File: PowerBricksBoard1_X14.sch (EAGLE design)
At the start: 16 parts

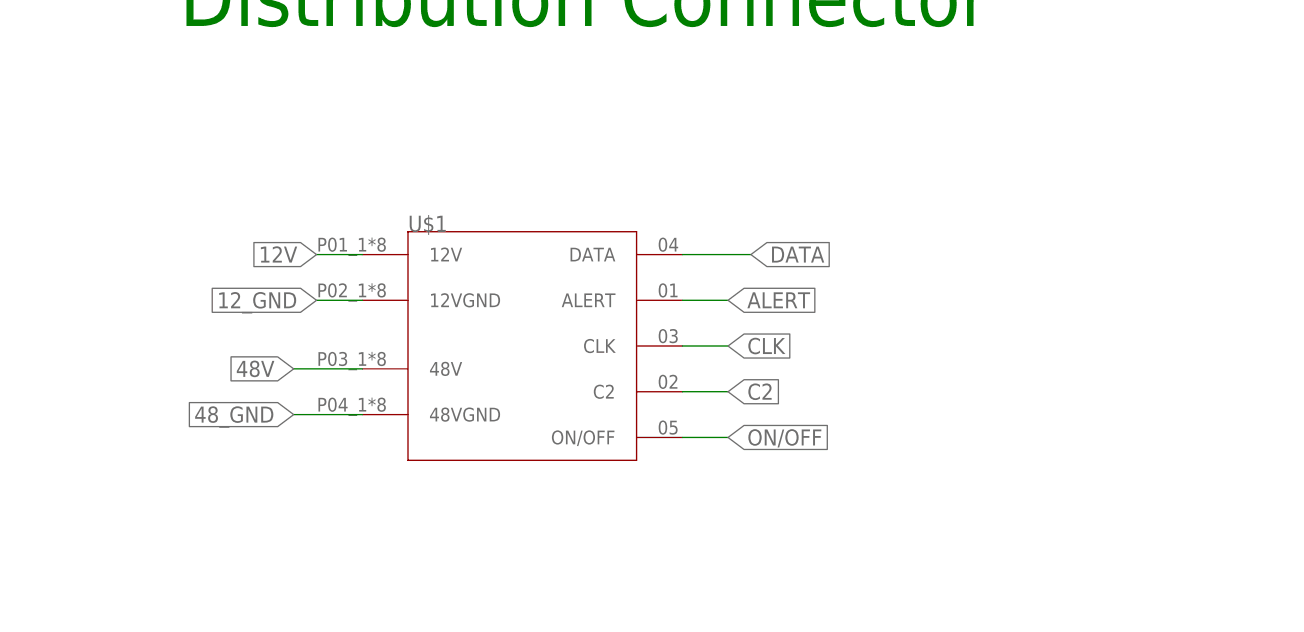
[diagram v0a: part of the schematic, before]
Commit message: more adjustments
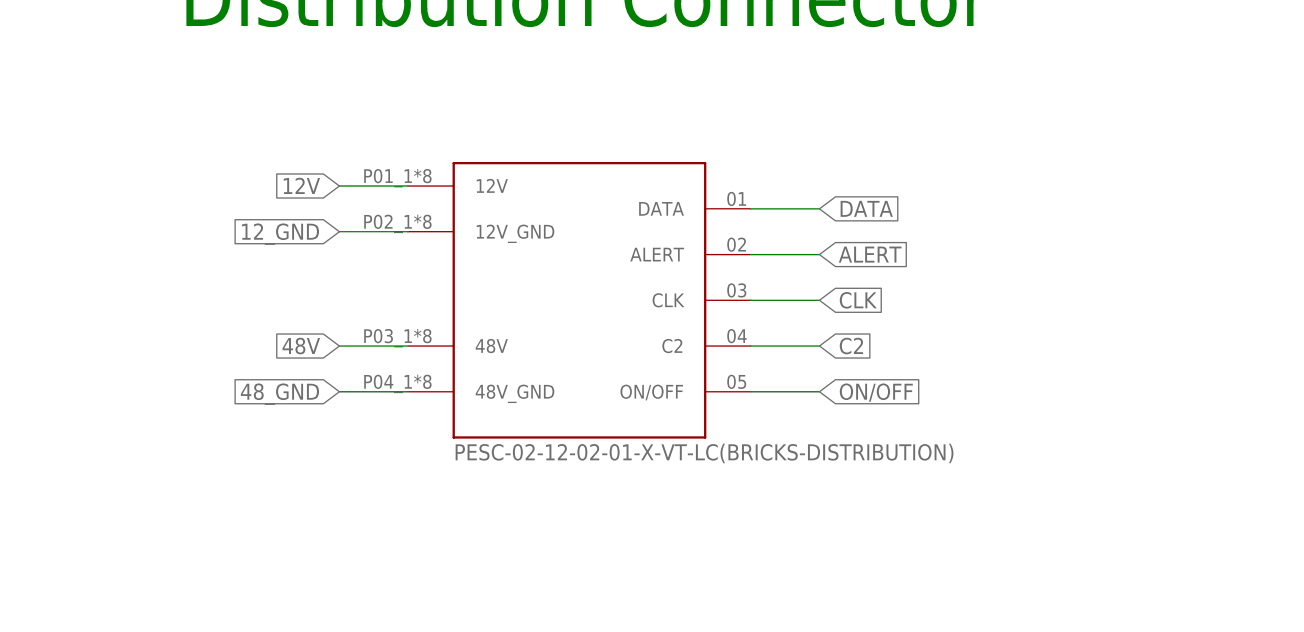
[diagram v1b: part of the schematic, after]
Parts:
- removed U$1: CONN_BRICKS, CONN, Distribution-Bricks:CONN_BRICKS
- added J1: PESC-02-12-02-01-X-VT-LC(BRICKS-DISTRIBUTION), CONN, Distribution-Bricks:PESC-02-12-02-01-X-VT-LC(BRICKS-DISTRIBUTION)
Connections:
- net 12V: now also J1.12V; no longer U$1.12V
- net 12_GND: now also J1.12V_GND; no longer U$1.12VGND
- net 48V: now also J1.48V; no longer U$1.48V
- net 48_GND: now also J1.48V_GND; no longer U$1.48VGND
- net ALERT: now also J1.ALERT; no longer U$1.ALERT
- net C2: now also J1.C2; no longer U$1.C2
- net CLK: now also J1.CLK; no longer U$1.CLK
- net DATA: now also J1.DATA; no longer U$1.DATA
- net ON/OFF: now also J1.ON/OFF; no longer U$1.ON/OFF
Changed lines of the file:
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@@
 <?xml version="1.0" encoding="utf-8"?>
 <!DOCTYPE eagle SYSTEM "eagle.dtd">
-<eagle version="9.6.2">
+<eagle version="9.5.0">
 <drawing>
 <settings>
@@
 <part name="R3" library="SparkFun-Resistors" library_urn="urn:adsk.eagle:library:532" deviceset="RESISTOR" device="0603" package3d_urn="urn:adsk.eagle:package:39650/1" value=" "/>
 <part name="R5" library="SparkFun-Resistors" library_urn="urn:adsk.eagle:library:532" deviceset="RESISTOR" device="0603" package3d_urn="urn:adsk.eagle:package:39650/1" value="510k"/>
-<part name="U$1" library="CONN, Distribution-Bricks" deviceset="CONN_BRICKS" device=""/>
+<part name="J1" library="CONN, Distribution-Bricks" deviceset="PESC-02-12-02-01-X-VT-LC(BRICKS-DISTRIBUTION)" device=""/>
 </parts>
 <sheets>
@@
 <attribute name="VALUE" x="109.22" y="115.316" size="1.778" layer="96" font="vector" align="top-center"/>
 </instance>
-<instance part="U$1" gate="G$1" x="195.58" y="119.38" smashed="yes">
-<attribute name="NAME" x="182.88" y="132.08" size="1.778" layer="95"/>
+<instance part="J1" gate="G$1" x="200.66" y="124.46" smashed="yes">
+<attribute name="VALUE" x="187.96" y="106.68" size="1.778" layer="96"/>
 </instance>
 </instances>
@@
 </segment>
 <segment>
-<wire x1="177.8" y1="111.76" x2="170.18" y2="111.76" width="0.1524" layer="91"/>
-<label x="170.18" y="111.76" size="1.778" layer="95" rot="MR0" xref="yes"/>
-<pinref part="U$1" gate="G$1" pin="48VGND"/>
+<pinref part="J1" gate="G$1" pin="48V_GND"/>
+<wire x1="182.88" y1="114.3" x2="175.26" y2="114.3" width="0.1524" layer="91"/>
+<label x="175.26" y="114.3" size="1.778" layer="95" rot="R180" xref="yes"/>
 </segment>
 </net>
@@
 </segment>
 <segment>
-<wire x1="177.8" y1="129.54" x2="172.72" y2="129.54" width="0.1524" layer="91"/>
-<label x="172.72" y="129.54" size="1.778" layer="95" rot="R180" xref="yes"/>
-<pinref part="U$1" gate="G$1" pin="12V"/>
+<pinref part="J1" gate="G$1" pin="12V"/>
+<wire x1="182.88" y1="137.16" x2="175.26" y2="137.16" width="0.1524" layer="91"/>
+<label x="175.26" y="137.16" size="1.778" layer="95" rot="R180" xref="yes"/>
 </segment>
 </net>
@@
 </segment>
 <segment>
-<wire x1="213.36" y1="114.3" x2="218.44" y2="114.3" width="0.1524" layer="91"/>
-<label x="218.44" y="114.3" size="1.778" layer="95" xref="yes"/>
-<pinref part="U$1" gate="G$1" pin="C2"/>
+<pinref part="J1" gate="G$1" pin="C2"/>
+<wire x1="220.98" y1="119.38" x2="228.6" y2="119.38" width="0.1524" layer="91"/>
+<label x="228.6" y="119.38" size="1.778" layer="95" xref="yes"/>
 </segment>
 </net>
@@
 </segment>
 <segment>
-<wire x1="177.8" y1="124.46" x2="172.72" y2="124.46" width="0.1524" layer="91"/>
-<label x="172.72" y="124.46" size="1.778" layer="95" rot="R180" xref="yes"/>
-<pinref part="U$1" gate="G$1" pin="12VGND"/>
+<pinref part="J1" gate="G$1" pin="12V_GND"/>
+<wire x1="182.88" y1="132.08" x2="175.26" y2="132.08" width="0.1524" layer="91"/>
+<label x="175.26" y="132.08" size="1.778" layer="95" rot="R180" xref="yes"/>
 </segment>
 </net>
@@
 </segment>
 <segment>
-<wire x1="213.36" y1="124.46" x2="218.44" y2="124.46" width="0.1524" layer="91"/>
-<label x="218.44" y="124.46" size="1.778" layer="95" xref="yes"/>
-<pinref part="U$1" gate="G$1" pin="ALERT"/>
+<pinref part="J1" gate="G$1" pin="ALERT"/>
+<wire x1="220.98" y1="129.54" x2="228.6" y2="129.54" width="0.1524" layer="91"/>
+<label x="228.6" y="129.54" size="1.778" layer="95" xref="yes"/>
 </segment>
 </net>
@@
 </segment>
 <segment>
-<wire x1="213.36" y1="129.54" x2="220.98" y2="129.54" width="0.1524" layer="91"/>
-<label x="220.98" y="129.54" size="1.778" layer="95" xref="yes"/>
-<pinref part="U$1" gate="G$1" pin="DATA"/>
+<pinref part="J1" gate="G$1" pin="DATA"/>
+<wire x1="220.98" y1="134.62" x2="228.6" y2="134.62" width="0.1524" layer="91"/>
+<label x="228.6" y="134.62" size="1.778" layer="95" xref="yes"/>
 </segment>
 </net>
@@
 </segment>
 <segment>
-<wire x1="213.36" y1="119.38" x2="218.44" y2="119.38" width="0.1524" layer="91"/>
-<label x="218.44" y="119.38" size="1.778" layer="95" xref="yes"/>
-<pinref part="U$1" gate="G$1" pin="CLK"/>
+<pinref part="J1" gate="G$1" pin="CLK"/>
+<wire x1="220.98" y1="124.46" x2="228.6" y2="124.46" width="0.1524" layer="91"/>
+<label x="228.6" y="124.46" size="1.778" layer="95" xref="yes"/>
 </segment>
 </net>
@@
 </segment>
 <segment>
-<wire x1="213.36" y1="109.22" x2="218.44" y2="109.22" width="0.1524" layer="91"/>
-<label x="218.44" y="109.22" size="1.778" layer="95" xref="yes"/>
-<pinref part="U$1" gate="G$1" pin="ON/OFF"/>
+<pinref part="J1" gate="G$1" pin="ON/OFF"/>
+<wire x1="220.98" y1="114.3" x2="228.6" y2="114.3" width="0.1524" layer="91"/>
+<label x="228.6" y="114.3" size="1.778" layer="95" xref="yes"/>
 </segment>
 </net>
@@
 </segment>
 <segment>
-<wire x1="177.8" y1="116.84" x2="170.18" y2="116.84" width="0.1524" layer="91"/>
-<label x="170.18" y="116.84" size="1.778" layer="95" rot="MR0" xref="yes"/>
-<pinref part="U$1" gate="G$1" pin="48V"/>
-</segment>
-<segment>
 <pinref part="U$2" gate="G$1" pin="VIN(+)"/>
 <wire x1="60.96" y1="127" x2="55.88" y2="127" width="0.1524" layer="91"/>
 <label x="55.88" y="127" size="1.778" layer="95" rot="R180" xref="yes"/>
 </segment>
-</net>
+<segment>
+<pinref part="J1" gate="G$1" pin="48V"/>
+<wire x1="182.88" y1="119.38" x2="175.26" y2="119.38" width="0.1524" layer="91"/>
+<label x="175.26" y="119.38" size="1.778" layer="95" rot="R180" xref="yes"/>
+</segment>
+</net>
